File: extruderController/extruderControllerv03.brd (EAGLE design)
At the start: 93.7 x 69.3 mm, 74 parts, among them IC1 LM1117MPX-5.0, IC2 MAX3467CPA, IC3 ATMEGA2561-16AU, IC4 ULN2003AD, J8 615016137621, Q2 PH7030L, Q3 PH7030L, Q4 PH7030L, Q5 PH7030L, Q6 PH7030L, X1 22-23-2081, X2 22-23-2081, X3 22-23-2101, X6 22-23-2041, X8 22-23-2031, X9 22-23-2031

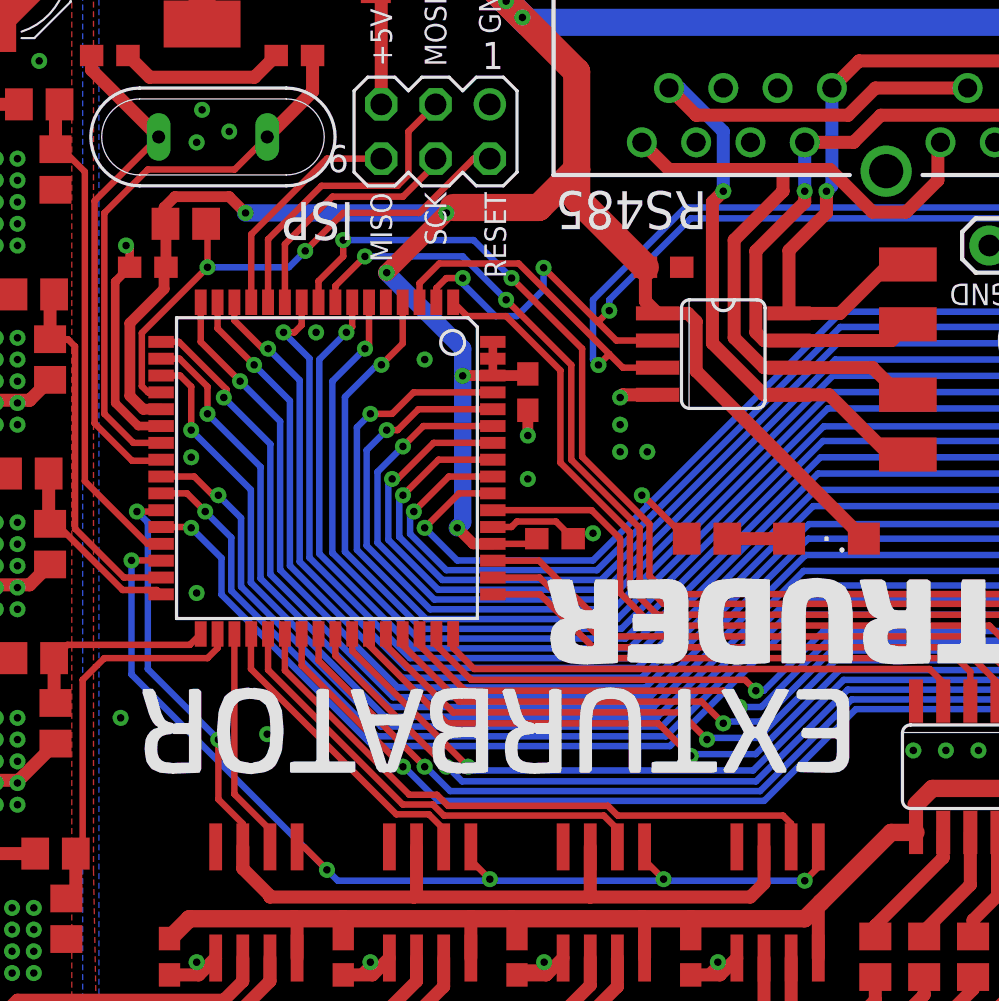
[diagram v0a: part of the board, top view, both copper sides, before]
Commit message: g
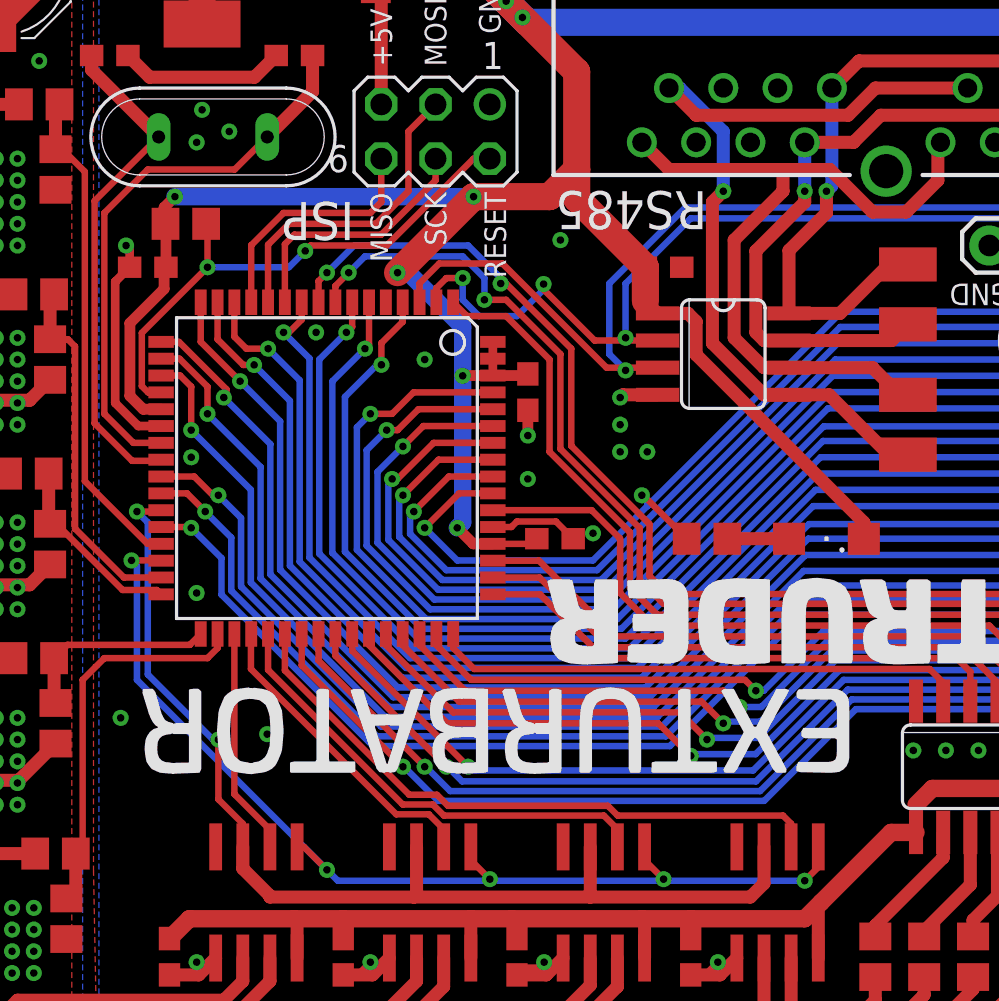
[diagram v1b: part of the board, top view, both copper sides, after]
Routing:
- net PB3(MISO): track 10.7 -> 11.6 mm
- net PE7: track 68.4 -> 67.6 mm
- net PE6: track 72.2 -> 72.8 mm
- net GND: vias 113 -> 114
